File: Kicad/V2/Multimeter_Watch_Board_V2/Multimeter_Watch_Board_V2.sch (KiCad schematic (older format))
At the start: 59 parts, among them J1 S3B-PH-K-S(LF)(SN), J2 S3B-PH-K-S(LF)(SN), J3 S3B-PH-K-S(LF)(SN), J6 51281-1294, J7 Conn_01x11_Female, J8 Conn_01x11_Female, Q1 A03400A N-MOS, U1 PCF85163-SO08, U2 AD8592, Y1 32kHz

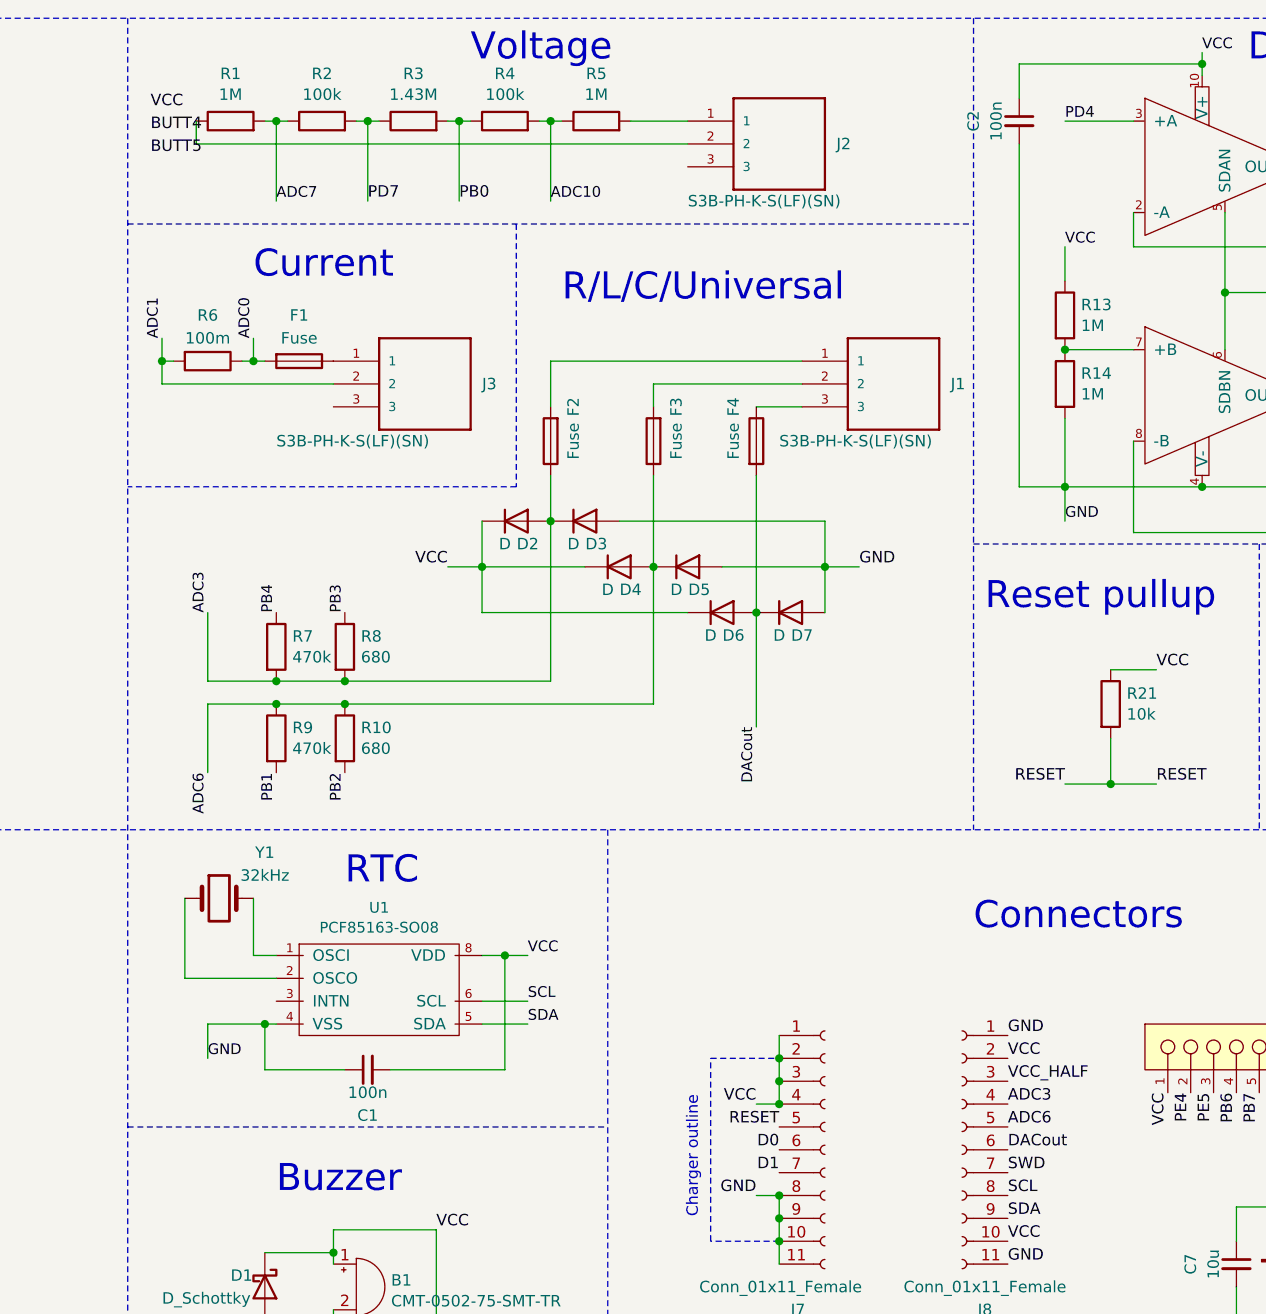
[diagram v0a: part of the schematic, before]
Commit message: implement rlc protection (likely to be reverted)
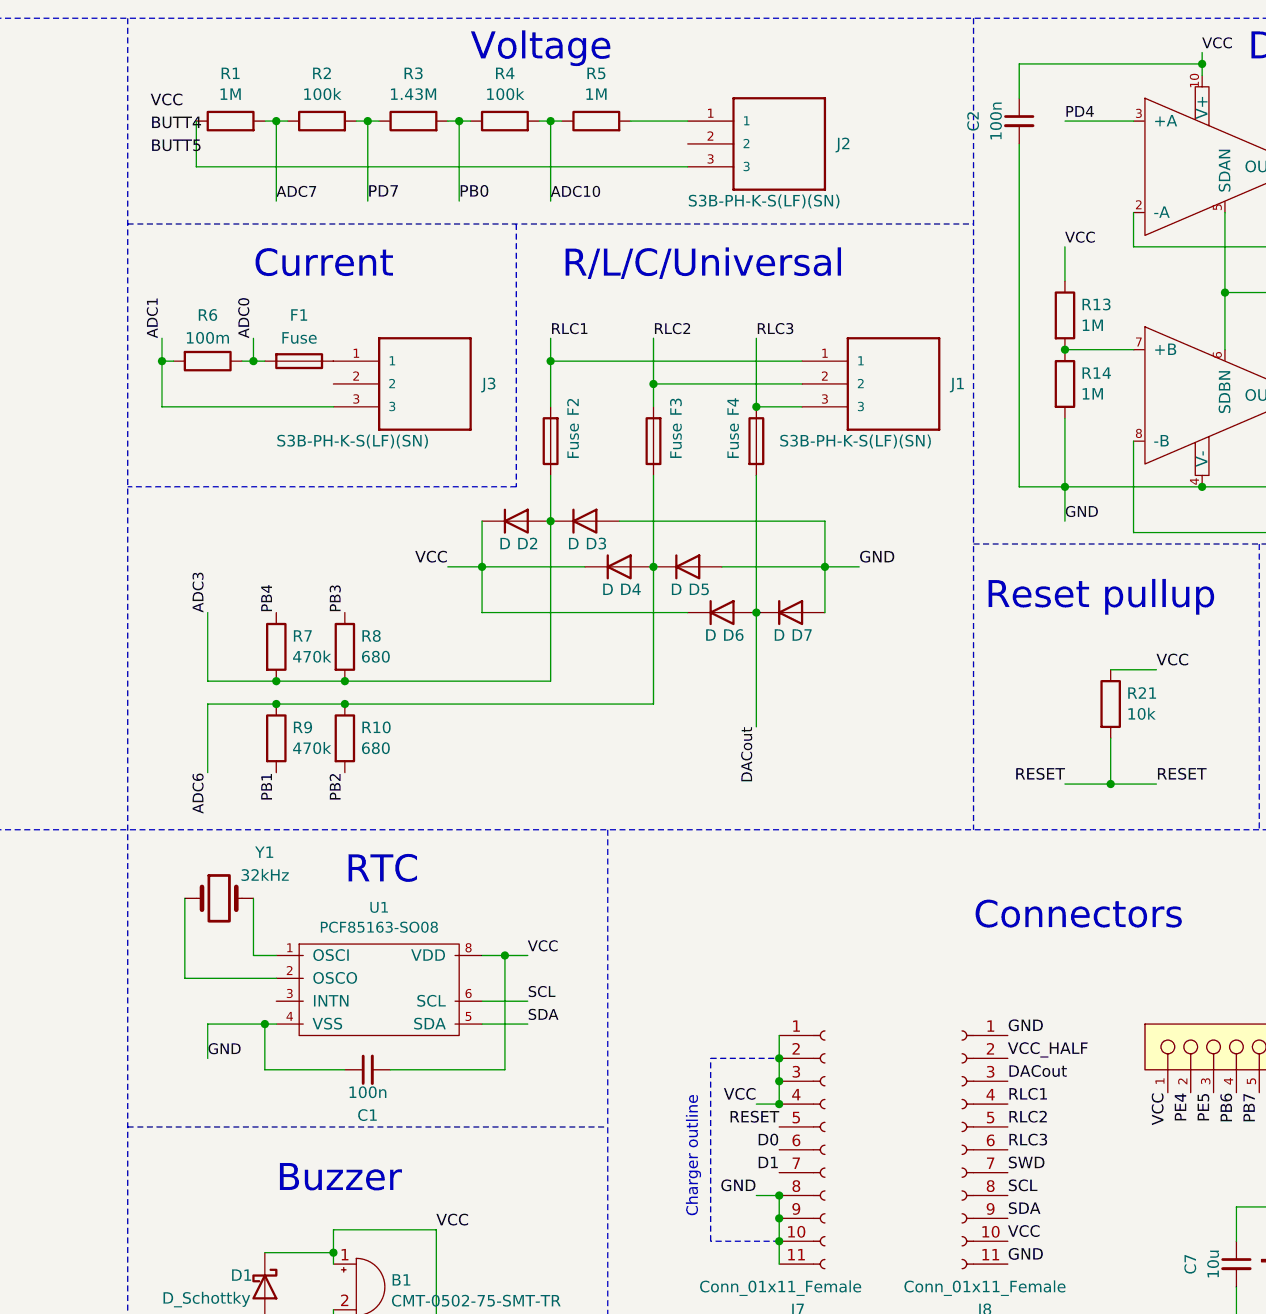
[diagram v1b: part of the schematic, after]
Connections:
- net ADC1: now also J3.3; no longer J3.2
- net ADC3: no longer J8.4 (Pin_4)
- net ADC6: no longer J8.5 (Pin_5)
- net DACout: now also J8.3 (Pin_3); no longer J8.6 (Pin_6)
- net VCC: no longer J8.2 (Pin_2)
- net VCC_HALF: now also J8.2 (Pin_2); no longer J8.3 (Pin_3)
- net at R1.1: now also J2.3; no longer J2.2
- net RLC1: now reaches F2.2, J1.1
- net RLC1: now also J8.4 (Pin_4)
- net RLC2: now reaches F3.2, J1.2
- net RLC2: now also J8.5 (Pin_5)
- net RLC3: now reaches F4.1, J1.3
- net RLC3: now also J8.6 (Pin_6)
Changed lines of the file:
@@
 Wire Wire Line
 	6700 950  6750 950
-Wire Wire Line
-	5200 950  5200 1050
 $Comp
 L Device:R R2
@@
 Text Label 10900 900  1    47   ~ 0
 ADC3
-Text Notes 6800 1750 0    118  ~ 0
+Text Notes 6800 1650 0    118  ~ 0
 R/L/C/Universal\n
-Wire Wire Line
-	5050 2000 5050 2100
 Text Label 7650 3600 3    47   ~ 0
 DACout
@@
 Text Label 8750 4950 0    50   ~ 0
 GND
-Text Label 8750 5150 0    50   ~ 0
+Text Label 8750 5050 0    50   ~ 0
 VCC_HALF
 Text Label 8750 5450 0    50   ~ 0
-DACout
+RLC3
 Text Label 8750 5550 0    50   ~ 0
 SWD
 Text Label 8750 5350 0    50   ~ 0
-ADC6
+RLC2
 Text Label 8750 5250 0    50   ~ 0
-ADC3
+RLC1
 Text Label 5950 1300 0    50   ~ 0
 PD7
@@
 Wire Wire Line
 	5450 2000 5400 2000
-Wire Wire Line
-	5050 2100 5800 2100
 Text Label 6350 1300 0    50   ~ 0
 PB0
-Wire Wire Line
-	5200 1050 7350 1050
 Wire Wire Line
 	7350 950  7100 950
@@
 Text Label 10250 5200 3    50   ~ 0
 GND
-Text Label 8750 5050 0    50   ~ 0
-VCC
 Text Label 9450 5200 3    50   ~ 0
 VCC
@@
 Wire Notes Line
 	4900 5350 7000 5350
+Wire Wire Line
+	7350 1150 5200 1150
+Wire Wire Line
+	5200 950  5200 1150
+Wire Wire Line
+	5800 2200 5050 2200
+Wire Wire Line
+	5050 2000 5050 2200
+Wire Wire Line
+	7200 2100 7200 1900
+Connection ~ 7200 2100
+Wire Wire Line
+	7650 2200 7650 1900
+Connection ~ 7650 2200
+Wire Wire Line
+	6750 2000 6750 1900
+Connection ~ 6750 2000
+Text Label 7650 1900 0    47   ~ 0
+RLC3
+Text Label 8750 5150 0    50   ~ 0
+DACout
+Text Label 7200 1900 0    47   ~ 0
+RLC2
+Text Label 6750 1900 0    47   ~ 0
+RLC1
 $EndSCHEMATC

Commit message: Revert "implement rlc protection (likely to be reverted)"
This reverts commit 3bbffdcc62f9ba327af4a0488dca8880d003efb7.
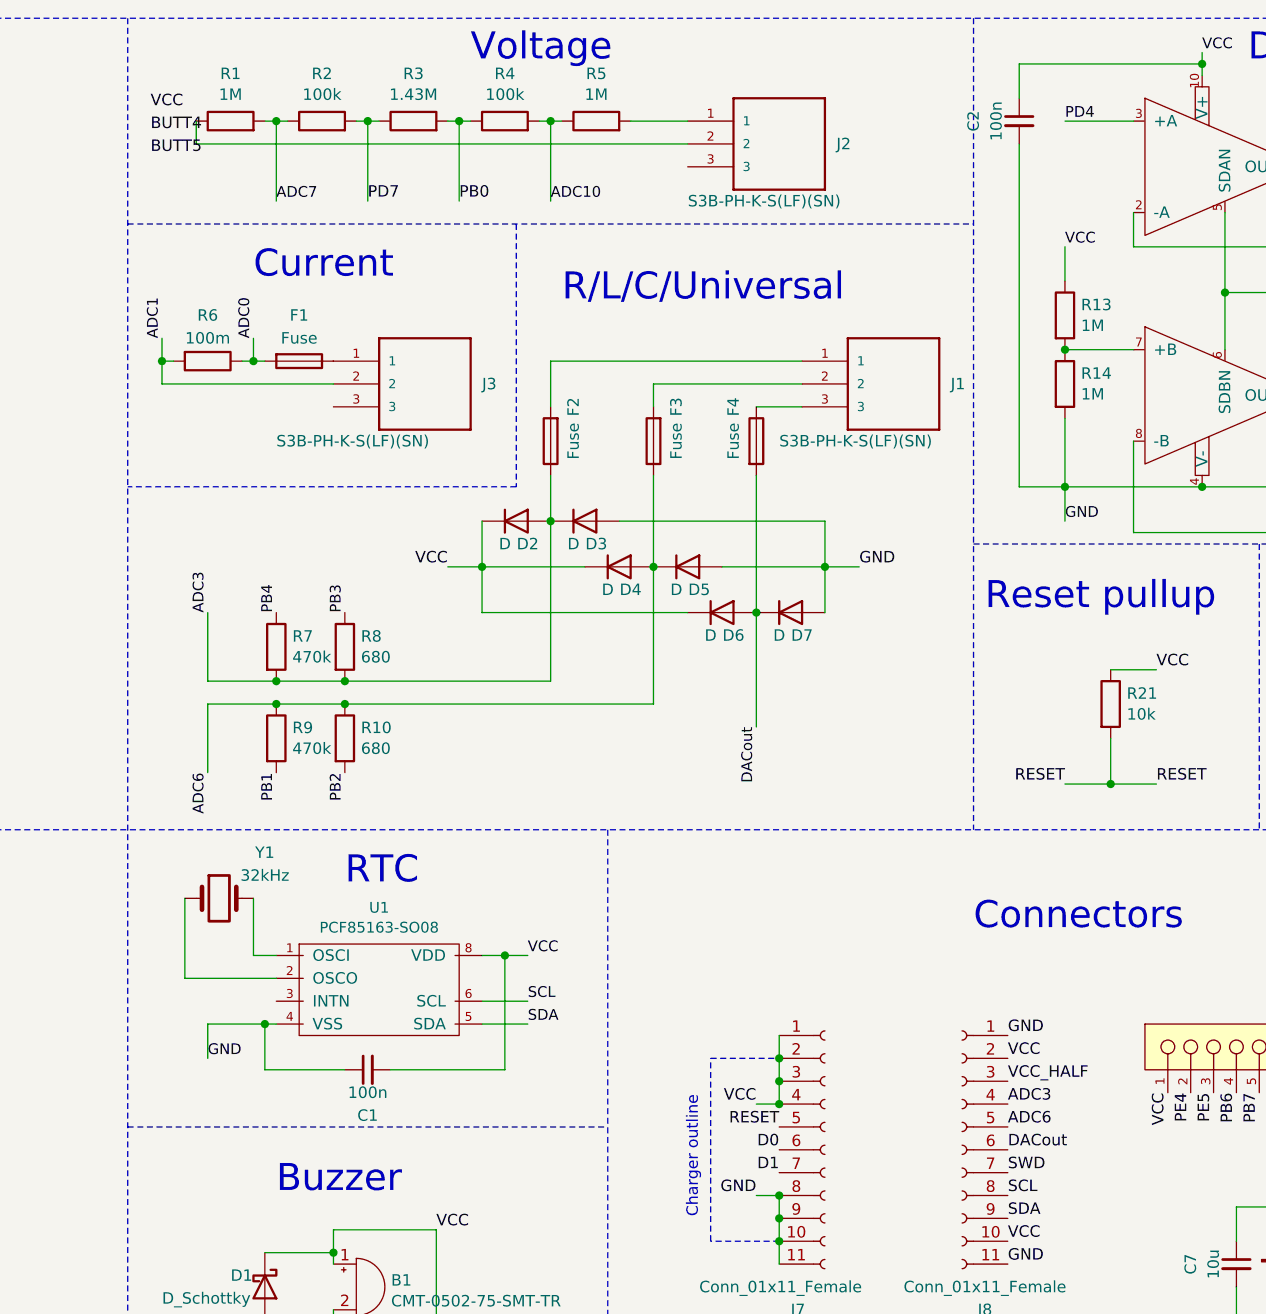
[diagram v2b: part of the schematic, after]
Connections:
- net ADC1: now also J3.2; no longer J3.3
- net ADC3: now also J8.4 (Pin_4)
- net ADC6: now also J8.5 (Pin_5)
- net DACout: now also J8.6 (Pin_6); no longer J8.3 (Pin_3)
- net VCC: now also J8.2 (Pin_2)
- net VCC_HALF: now also J8.3 (Pin_3); no longer J8.2 (Pin_2)
- net at R1.1: now also J2.2; no longer J2.3
- net RLC1: no longer names the net of F2.2, J1.1
- net RLC1: no longer J8.4 (Pin_4)
- net RLC2: no longer names the net of F3.2, J1.2
- net RLC2: no longer J8.5 (Pin_5)
- net RLC3: no longer names the net of F4.1, J1.3
- net RLC3: no longer J8.6 (Pin_6)
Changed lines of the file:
@@
 Wire Wire Line
 	6700 950  6750 950
+Wire Wire Line
+	5200 950  5200 1050
 $Comp
 L Device:R R2
@@
 Text Label 10900 900  1    47   ~ 0
 ADC3
-Text Notes 6800 1650 0    118  ~ 0
+Text Notes 6800 1750 0    118  ~ 0
 R/L/C/Universal\n
+Wire Wire Line
+	5050 2000 5050 2100
 Text Label 7650 3600 3    47   ~ 0
 DACout
@@
 Text Label 8750 4950 0    50   ~ 0
 GND
-Text Label 8750 5050 0    50   ~ 0
+Text Label 8750 5150 0    50   ~ 0
 VCC_HALF
 Text Label 8750 5450 0    50   ~ 0
-RLC3
+DACout
 Text Label 8750 5550 0    50   ~ 0
 SWD
 Text Label 8750 5350 0    50   ~ 0
-RLC2
+ADC6
 Text Label 8750 5250 0    50   ~ 0
-RLC1
+ADC3
 Text Label 5950 1300 0    50   ~ 0
 PD7
@@
 Wire Wire Line
 	5450 2000 5400 2000
+Wire Wire Line
+	5050 2100 5800 2100
 Text Label 6350 1300 0    50   ~ 0
 PB0
+Wire Wire Line
+	5200 1050 7350 1050
 Wire Wire Line
 	7350 950  7100 950
@@
 Text Label 10250 5200 3    50   ~ 0
 GND
+Text Label 8750 5050 0    50   ~ 0
+VCC
 Text Label 9450 5200 3    50   ~ 0
 VCC
@@
 Wire Notes Line
 	4900 5350 7000 5350
-Wire Wire Line
-	7350 1150 5200 1150
-Wire Wire Line
-	5200 950  5200 1150
-Wire Wire Line
-	5800 2200 5050 2200
-Wire Wire Line
-	5050 2000 5050 2200
-Wire Wire Line
-	7200 2100 7200 1900
-Connection ~ 7200 2100
-Wire Wire Line
-	7650 2200 7650 1900
-Connection ~ 7650 2200
-Wire Wire Line
-	6750 2000 6750 1900
-Connection ~ 6750 2000
-Text Label 7650 1900 0    47   ~ 0
-RLC3
-Text Label 8750 5150 0    50   ~ 0
-DACout
-Text Label 7200 1900 0    47   ~ 0
-RLC2
-Text Label 6750 1900 0    47   ~ 0
-RLC1
 $EndSCHEMATC
